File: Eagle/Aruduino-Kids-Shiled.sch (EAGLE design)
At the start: 16 parts

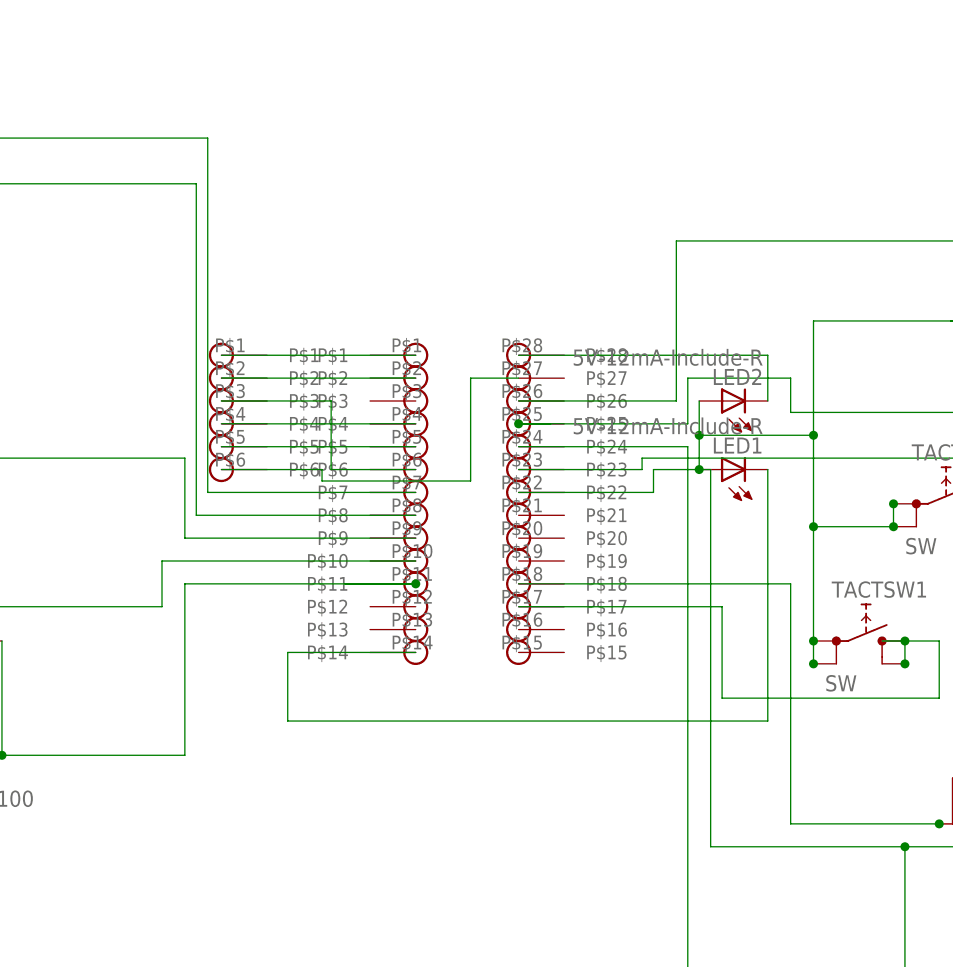
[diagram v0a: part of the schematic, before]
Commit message: Second
few changes
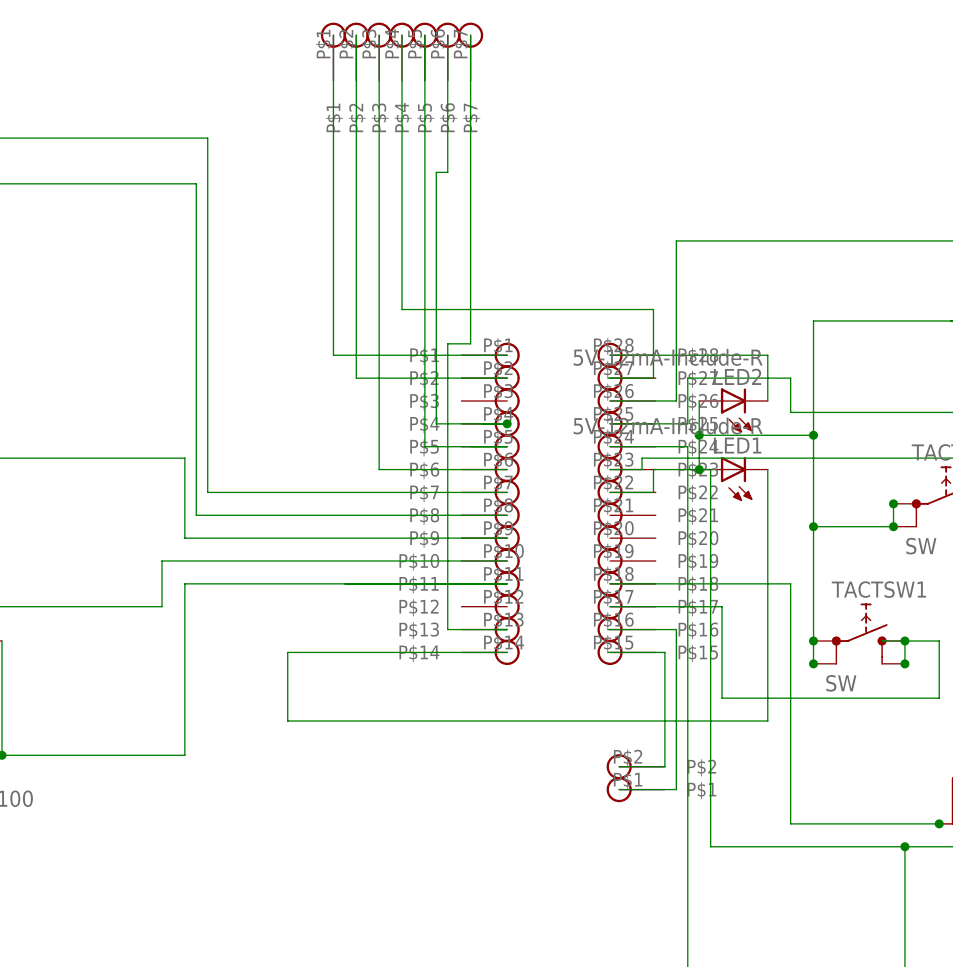
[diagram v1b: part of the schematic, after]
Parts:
- added U$3: SIPS-7, Aruduino-Kids-Shiled:SIPS-7
- U$6: value C-03784 -> SIPS-2; device Aruduino-Kids-Shiled:C-03784 -> Aruduino-Kids-Shiled:SIPS-2
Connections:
- new net N$25: U$1.P$13, U$3.P$7
- new net N$26: U$1.P$16, U$6.P$1
- new net N$27: U$1.P$15, U$6.P$2
- net N$10: now also U$3.P$1; no longer U$6.P$1
- net N$12: now also U$3.P$4; no longer U$6.P$6
- net N$14: now also U$3.P$2; no longer U$6.P$2
- net N$15: now also U$3.P$3; no longer U$6.P$3
- net N$16: now also U$1.P$5, U$3.P$5; no longer U$1.P$4, U$6.P$4
- net N$17: now also U$1.P$4, U$3.P$6; no longer U$1.P$5, U$6.P$5

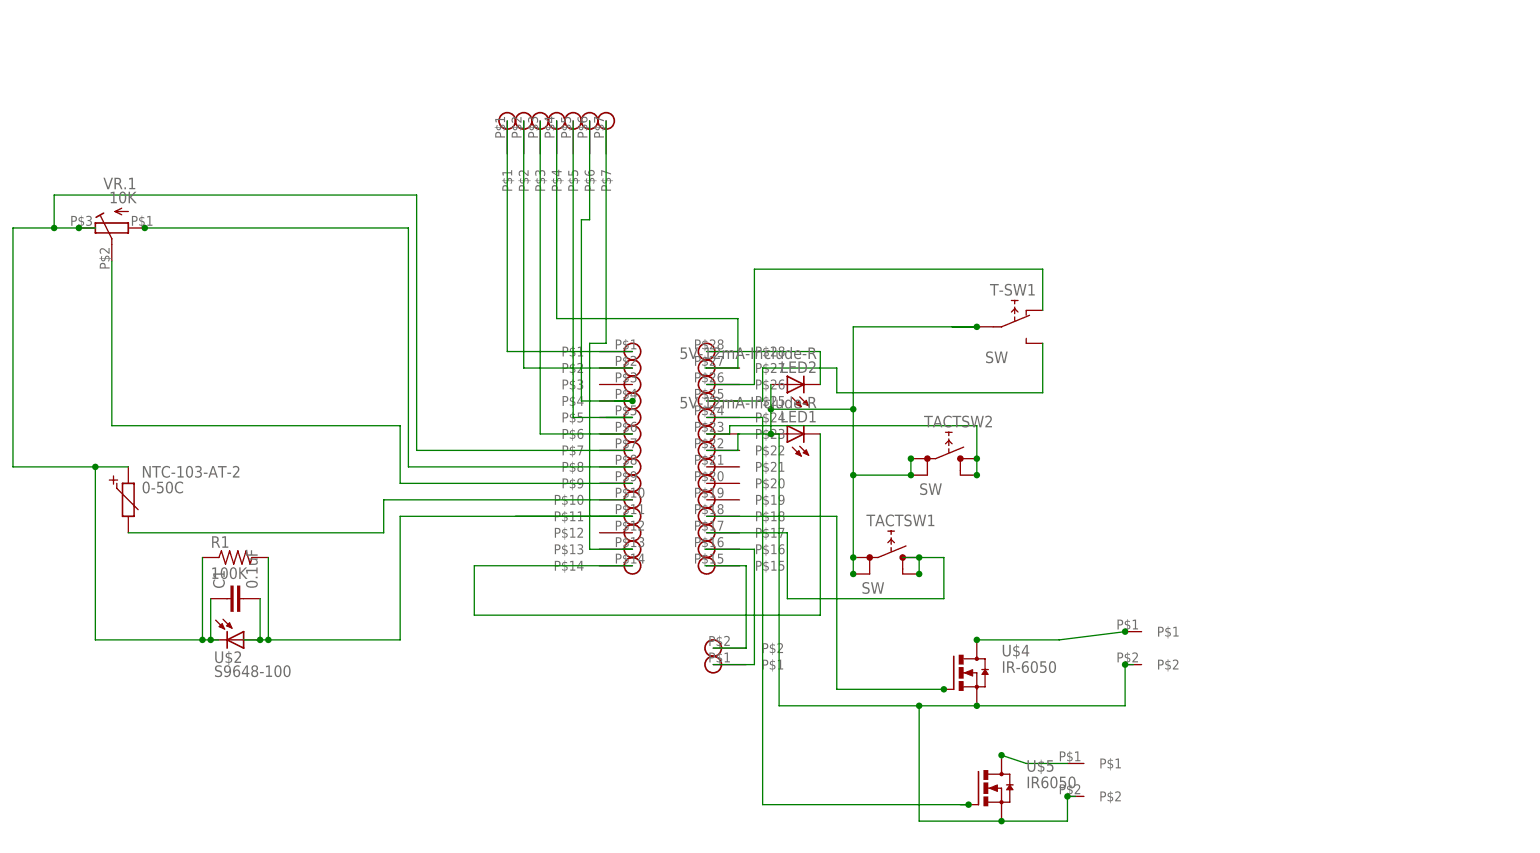
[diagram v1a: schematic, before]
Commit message: Semi_Final
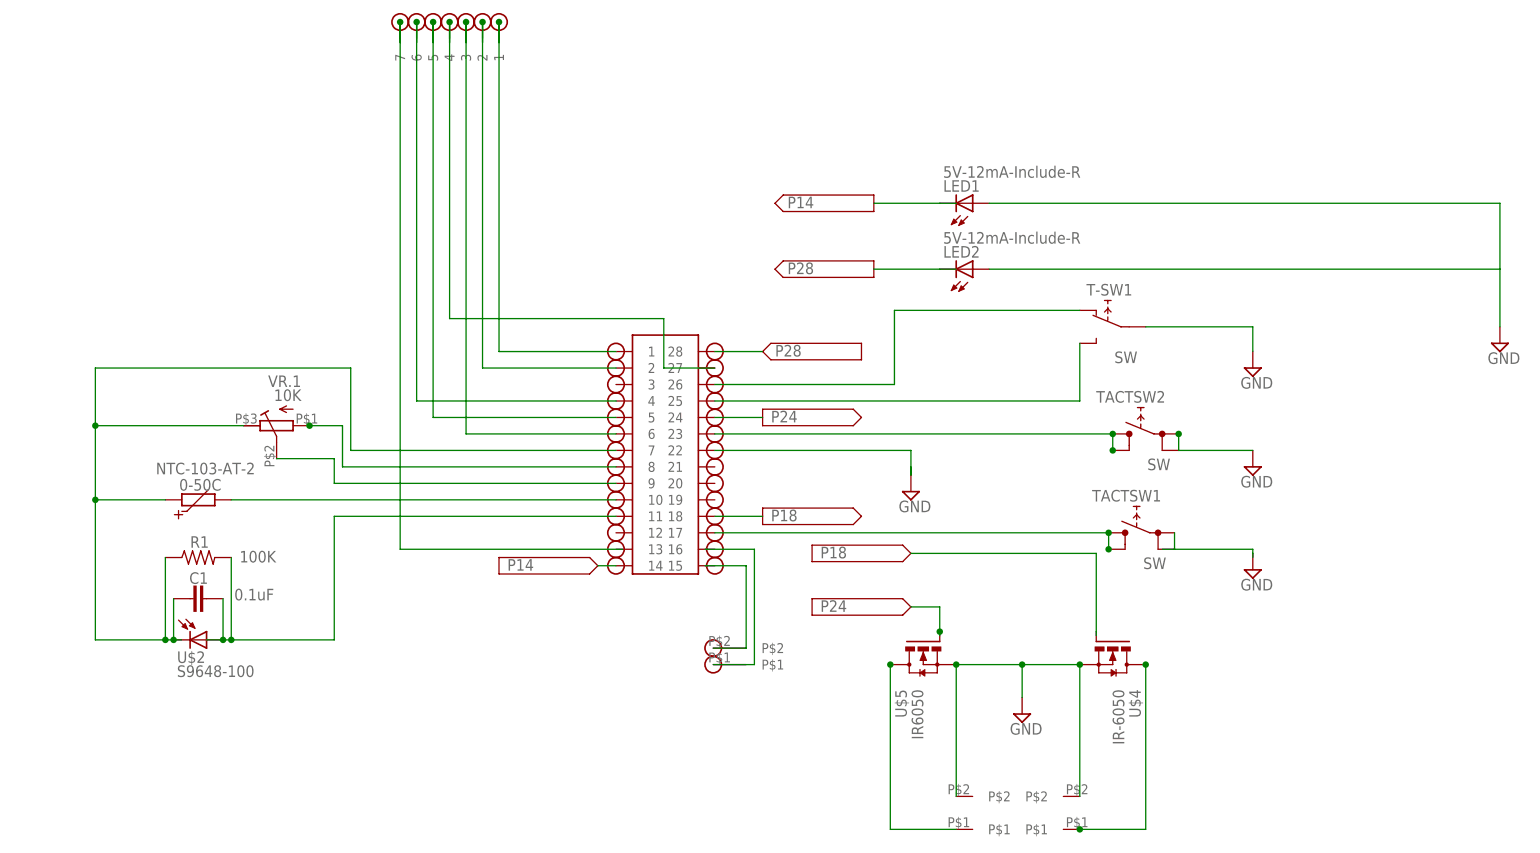
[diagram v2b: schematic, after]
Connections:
- removed net N$1: LED1.A, LED2.A, T-SW1.2COM, TACTSW1.1, TACTSW1.3, TACTSW2.1, TACTSW2.3, TB1.P$2, TB2.P$2, U$1.P$22, U$4.S, U$5.S
- removed net N$19: U$1.P$18, U$4.G
- removed net N$2: LED1.C, U$1.P$14
- removed net N$20: U$1.P$24, U$5.G
- removed net N$3: LED2.C, U$1.P$28
- new net GND: LED1.A, LED2.A, T-SW1.2COM, TACTSW1.1, TACTSW1.3, TACTSW2.1, TACTSW2.3, TB1.P$2, TB2.P$2, U$1.22, U$4.S, U$5.S
- new net P14: LED1.C, U$1.14
- new net P18: U$1.18, U$4.G
- new net P24: U$1.24, U$5.G
- new net P28: LED2.C, U$1.28
- net N$10: now also U$1.1, U$3.1; no longer U$1.P$1, U$3.P$1
- net N$11: now also U$1.23; no longer U$1.P$23
- net N$12: now also U$1.27, U$3.4; no longer U$1.P$27, U$3.P$4
- net N$13: now also U$1.25; no longer U$1.P$25
- net N$14: now also U$1.2, U$3.2; no longer U$1.P$2, U$3.P$2
- net N$15: now also U$1.6, U$3.3; no longer U$1.P$6, U$3.P$3
- net N$16: now also U$1.5, U$3.5; no longer U$1.P$5, U$3.P$5
- net N$17: now also U$1.4, U$3.6; no longer U$1.P$4, U$3.P$6
- net N$18: now also U$1.26; no longer U$1.P$26
- net N$25: now also U$1.13, U$3.7; no longer U$1.P$13, U$3.P$7
- net N$26: now also U$1.16; no longer U$1.P$16
- net N$27: now also U$1.15; no longer U$1.P$15
- net N$4: now also U$1.10; no longer U$1.P$10
- net N$5: now also U$1.11; no longer U$1.P$11
- net N$6: now also U$1.7; no longer U$1.P$7
- net N$7: now also U$1.8; no longer U$1.P$8
- net N$8: now also U$1.9; no longer U$1.P$9
- net N$9: now also U$1.17; no longer U$1.P$17
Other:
- moved on the sheet: 0-50C, C1, LED1, LED2, R1, T-SW1, TACTSW1, TACTSW2, U$2, U$4, U$5, VR.1

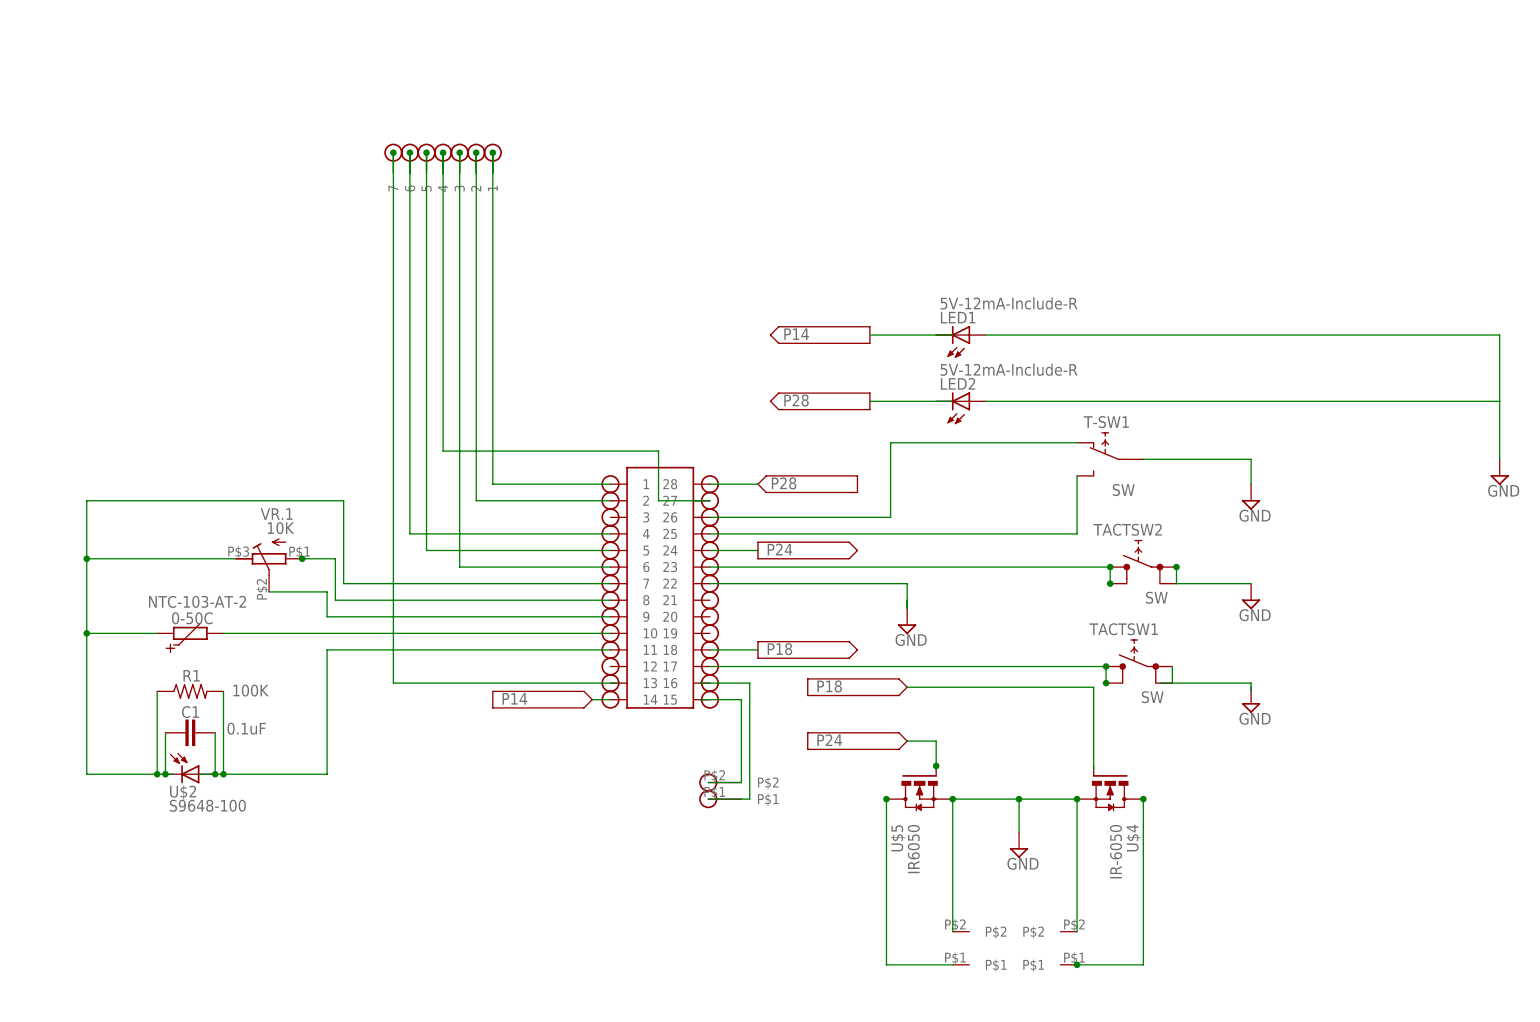
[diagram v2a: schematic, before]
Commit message: Practice-Final
Test-Build
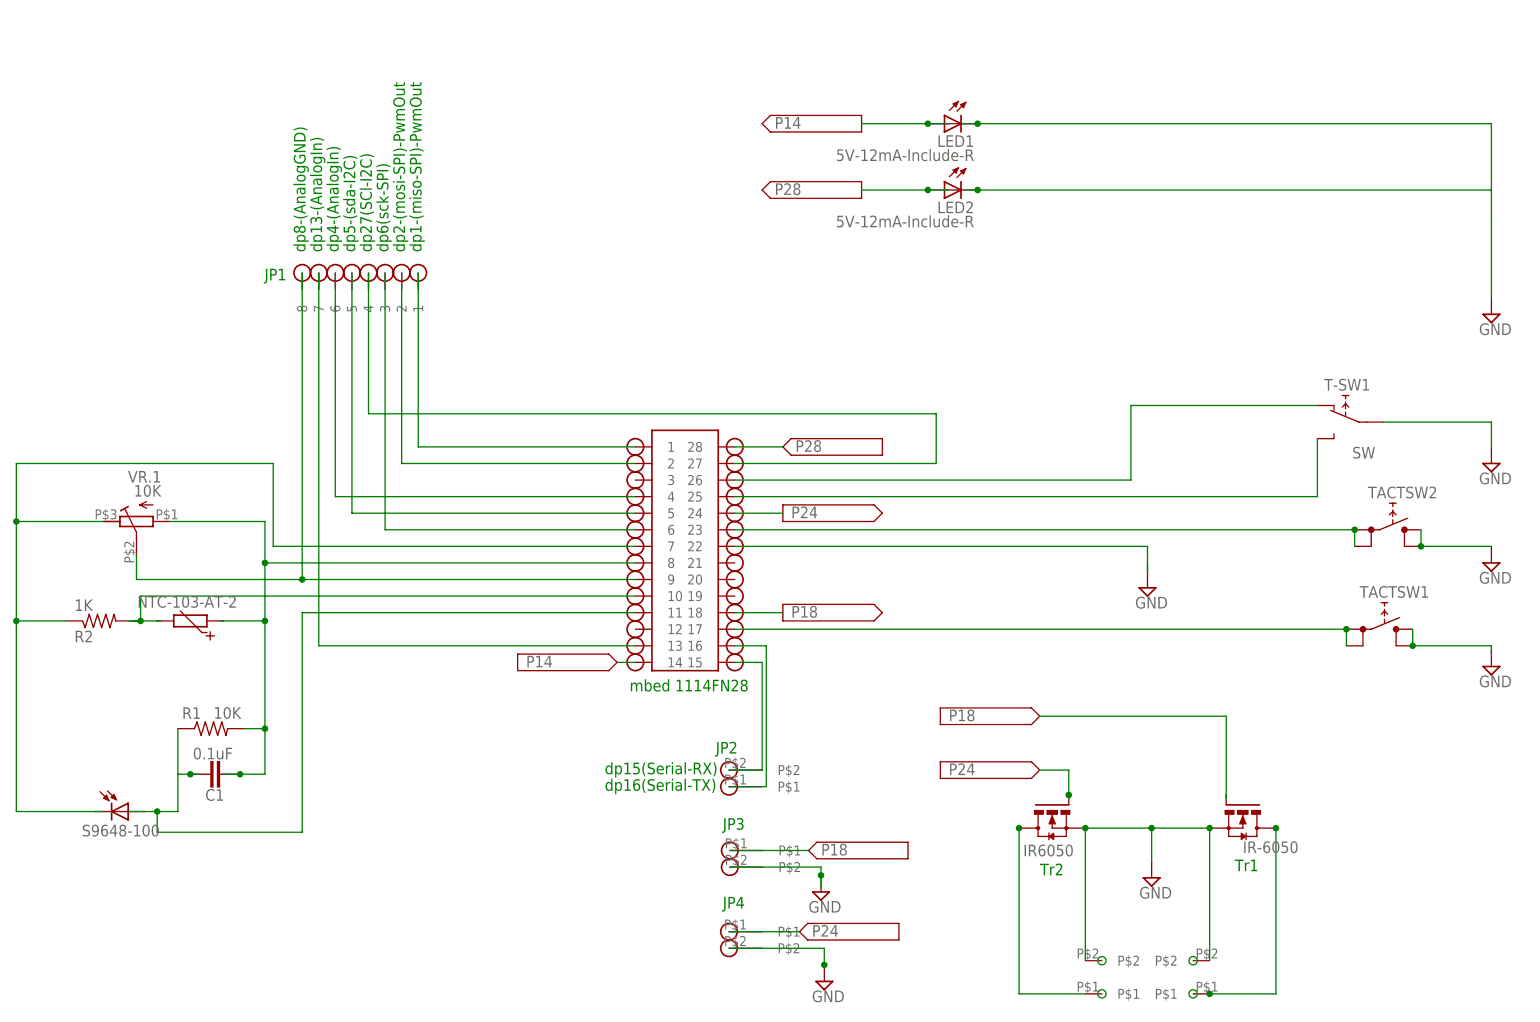
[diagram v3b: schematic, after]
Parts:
- added R2: 1K, Aruduino-Kids-Shiled:R
- added U$10, U$9: SIPS-2, Aruduino-Kids-Shiled:SIPS-2
- R1: value 100K -> 10K
- TACTSW1, TACTSW2: value SW -> (none)
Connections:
- removed net N$7: U$1.8, VR.1.A
- new net N$33: 0-50C.2, R2.2, U$1.10
- net GND: now also LED1.C, LED2.C, TACTSW1.2, TACTSW1.4, TACTSW2.2, TACTSW2.4, U$10.P$2, U$9.P$2; no longer LED1.A, LED2.A, TACTSW1.1, TACTSW1.3, TACTSW2.1, TACTSW2.3
- net N$11: now also TACTSW2.1, TACTSW2.3; no longer TACTSW2.2, TACTSW2.4
- net N$4: now also R2.1, U$1.7, U$2.C, VR.1.E; no longer 0-50C.2, U$1.10
- net N$5: now also R1.1; no longer R1.2
- net N$6: now also R1.2, U$1.8, VR.1.A; no longer R1.1, U$1.7, U$2.C, VR.1.E
- net N$8: now also U$3.8
- net N$9: now also TACTSW1.1, TACTSW1.3; no longer TACTSW1.2, TACTSW1.4
- net P14: now also LED1.A; no longer LED1.C
- net P18: now also U$10.P$1
- net P24: now also U$9.P$1
- net P28: now also LED2.A; no longer LED2.C
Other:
- note added: "JP1"
- note added: "JP2"
- note added: "JP3"
- note added: "JP4"
- note added: "Tr1"
- note added: "Tr2"
- note added: "dp1-(miso-SPI)-PwmOut"
- note added: "dp13-(AnalogIn)"
- note added: "dp15(Serial-RX)"
- note added: "dp16(Serial-TX)"
- note added: "dp2-(mosi-SPI)-PwmOut"
- note added: "dp27(SCl-I2C)"
- note added: "dp4-(AnalogIn)"
- note added: "dp5-(sda-I2C)"
- note added: "dp6(sck-SPI)"
- note added: "dp8-(AnalogGND)"
- note added: "mbed 1114FN28"
- moved on the sheet: C1, LED1, LED2, R1, T-SW1, VR.1
